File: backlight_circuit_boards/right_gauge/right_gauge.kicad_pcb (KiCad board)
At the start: 2 copper layers, 95 x 86 mm, 14 parts, among them J1 IN, J2 OUT

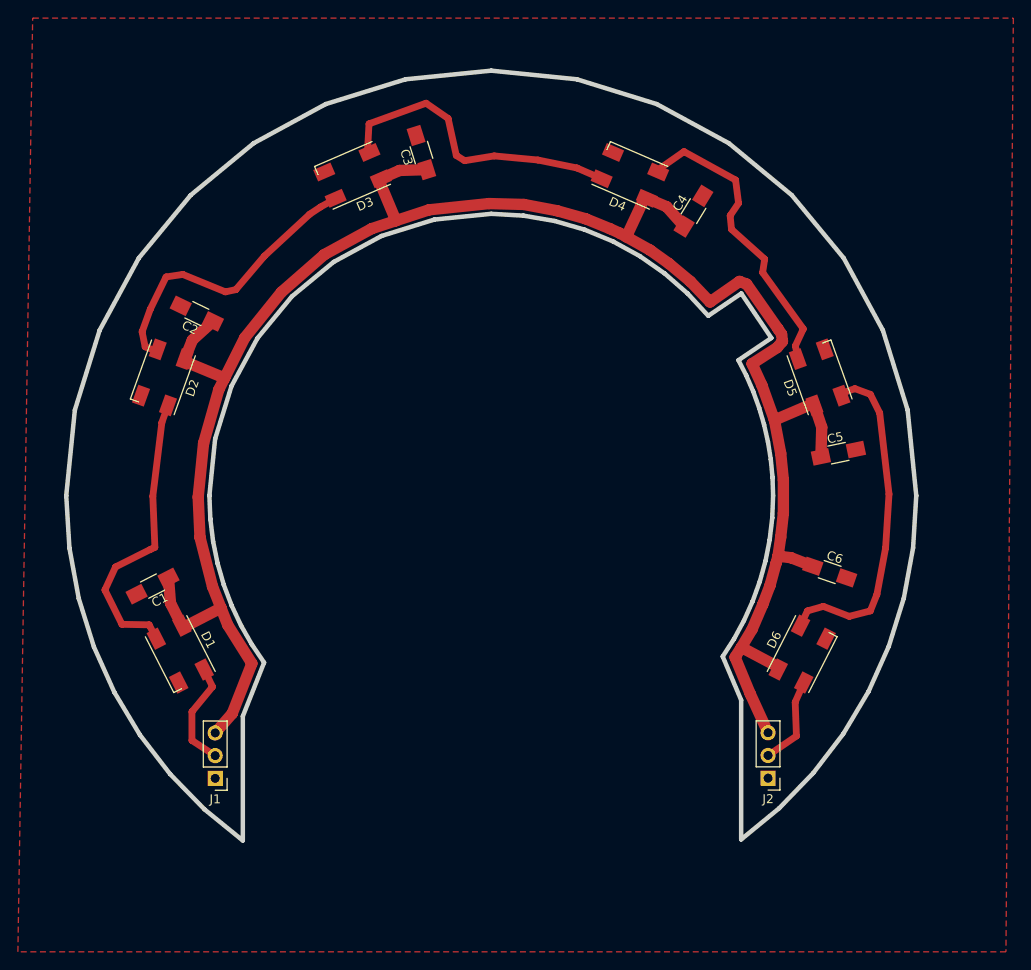
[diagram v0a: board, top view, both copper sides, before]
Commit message: improvements to all boards
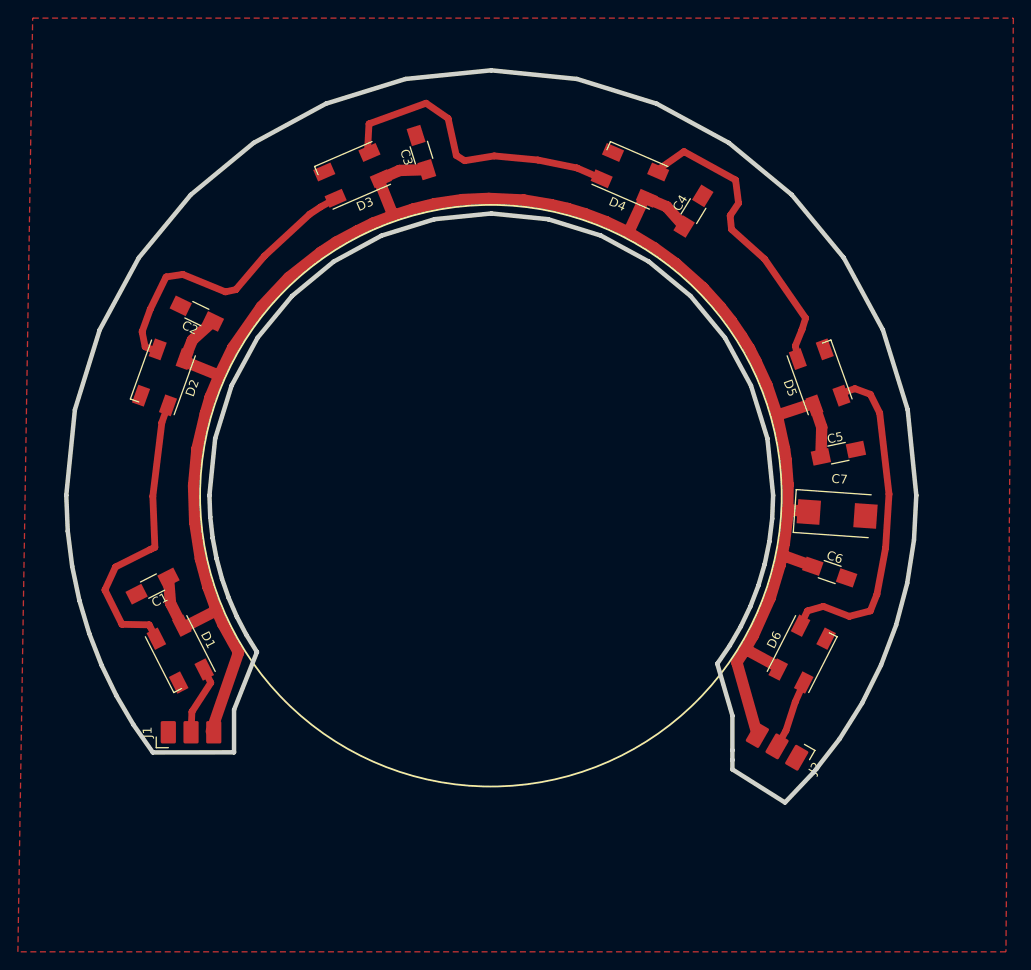
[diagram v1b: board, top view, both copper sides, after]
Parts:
- added C7: 10 uF, Capacitors_Tantalum_SMD:CP_Tantalum_Case-D_EIA-7343-31_Reflow, F.Cu at (121.5, 82.9)
- J1, J2: footprint Pin_Headers:Pin_Header_Straight_1x03_Pitch2.54mm -> Frickelbude Connectors:wire_solder_pads_1x03_2.5x1.7mm_Pitch2.54mm
- moved J1 7.35 mm to (46.8, 107.3), turned to 90 degrees
- moved J2 3.93 mm to (117.0, 110.1), turned to 240 degrees
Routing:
- net VCC: track 230.4 -> 220.5 mm
- net Net-(D1-Pad4): track 12.3 -> 8.07 mm
- net Net-(D6-Pad2): track 10.3 -> 8.01 mm
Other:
- board size 95 x 86 mm -> 95 x 81.8 mm
